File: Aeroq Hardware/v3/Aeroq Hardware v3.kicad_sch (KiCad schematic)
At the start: 63 parts, among them Q1 Si1308EDL, U2 ESP32-C3-MINI-1-N4, U3 AMS1117-3.3, U4 SCD40-D-R1

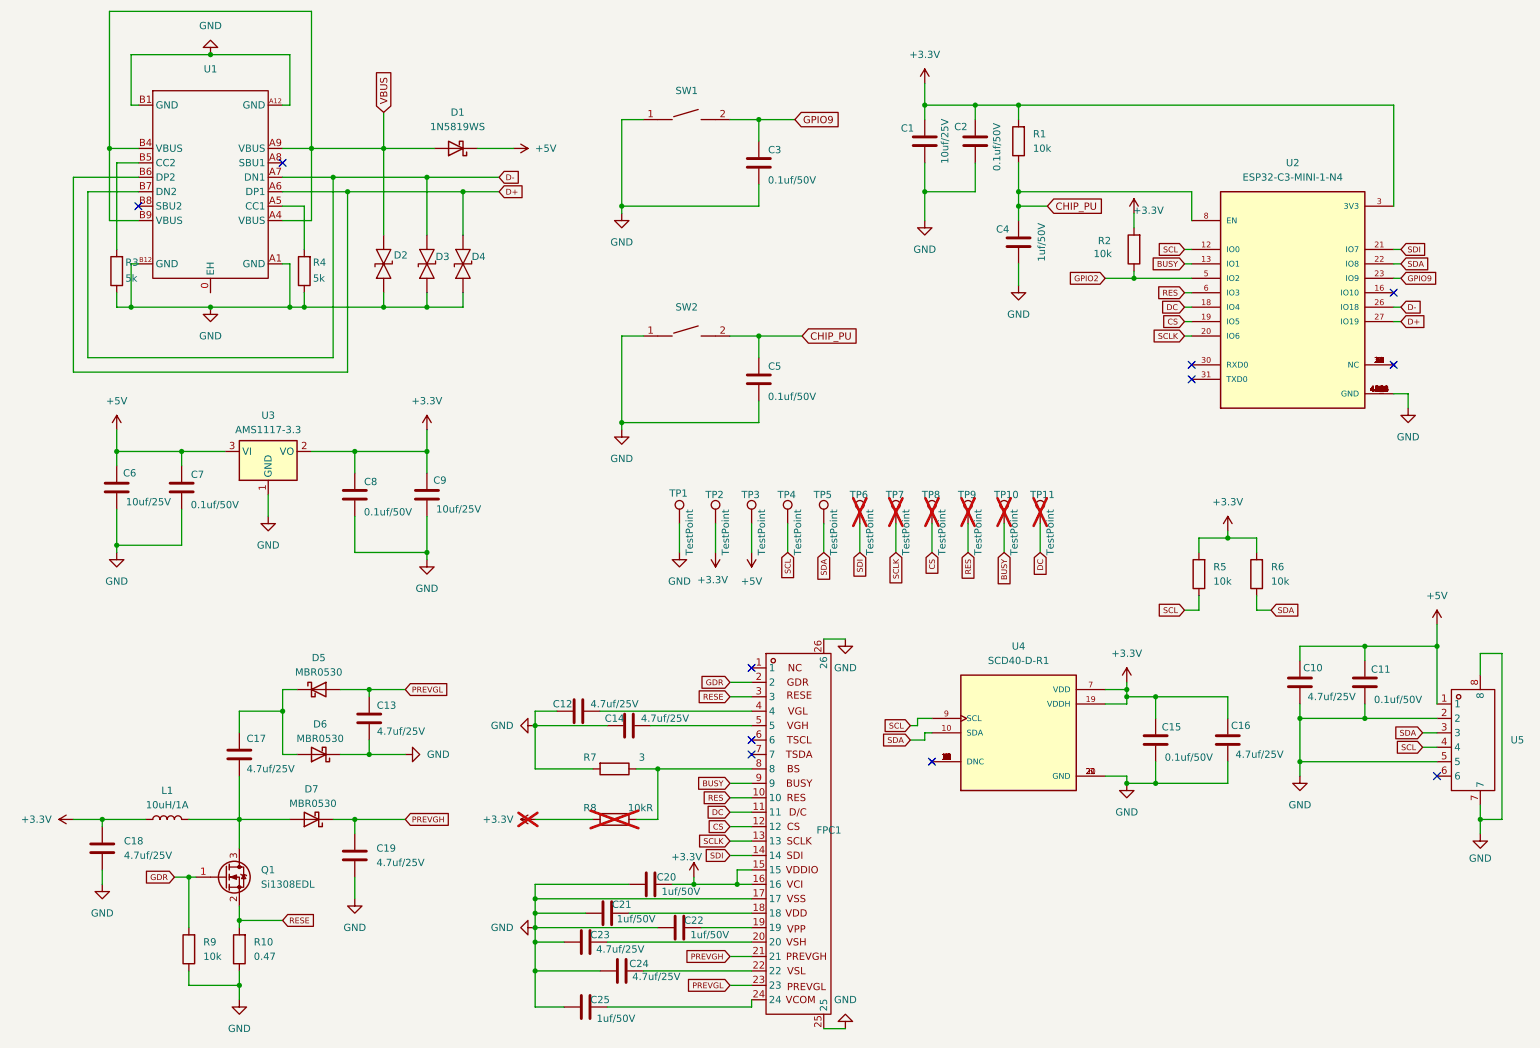
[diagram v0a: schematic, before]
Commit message: add my customizations
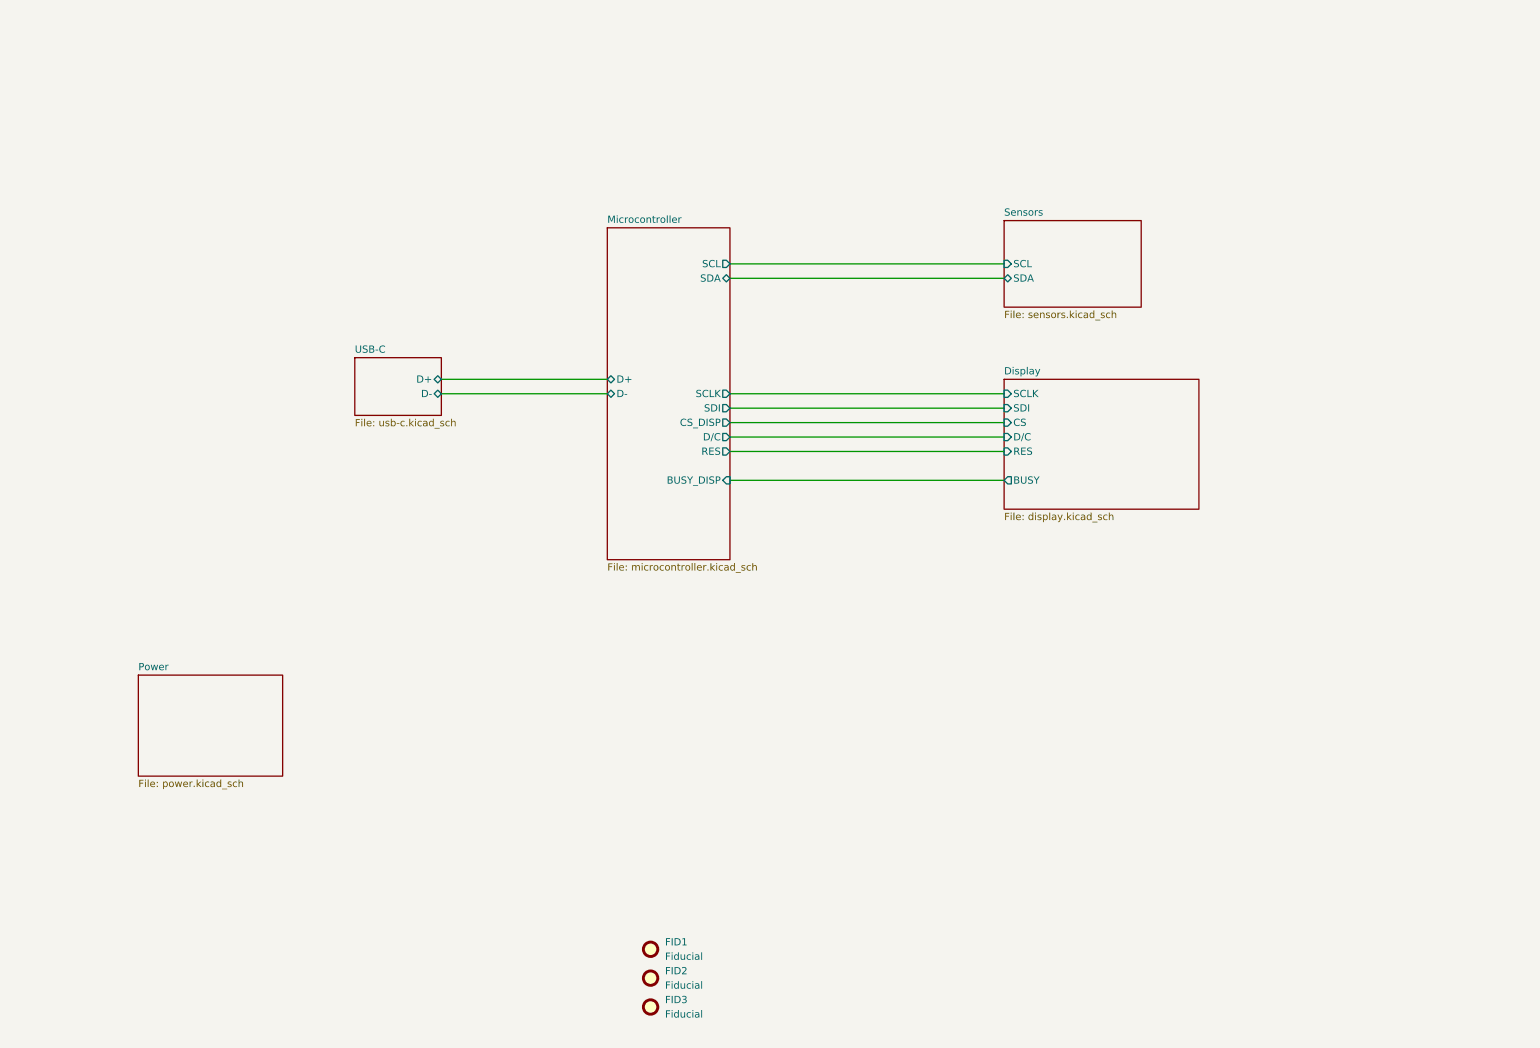
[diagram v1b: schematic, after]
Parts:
- removed C1, C6, C9: 10uf/25V, Capacitor_SMD:C_0603_1608Metric, symbol Device:C
- removed C10, C12, C13, C14, C16, C17, C18, C19, C23, C24: 4.7uf/25V, Capacitor_SMD:C_0603_1608Metric, symbol Device:C
- removed C11, C15, C2, C3, C5, C7, C8: 0.1uf/50V, Capacitor_SMD:C_0603_1608Metric, symbol Device:C
- removed C20, C21, C22, C25, C4: 1uf/50V, Capacitor_SMD:C_0603_1608Metric, symbol Device:C
- removed D1: 1N5819WS, Diode_SMD:D_SOD-323, symbol Diode:1N5819WS
- removed D2, D3, D4: ~, Project Footprints:SOD-523_L1.2-W0.8-LS1.6-BI, symbol LRC LESD5D5.0CT1G:LESD5D5.0CT1G
- removed D5, D6, D7: MBR0530, Diode_SMD:D_SOD-123, symbol Diode:MBR0530
- removed FPC1: ~, Project Footprints:FPC-SMD_24P-P0.50_FPC-05FB-24PH20, symbol FPC-05FB-24PH20:FPC-05FB-24PH20
- removed L1: 10uH/1A, Inductor_SMD:L_1210_3225Metric, symbol Device:L
- removed Q1: Si1308EDL, Package_TO_SOT_SMD:SOT-323_SC-70, symbol Transistor_FET:Si1308EDL
- removed R1, R2, R5, R6, R9: 10k, Resistor_SMD:R_0402_1005Metric, symbol Device:R
- removed R10: 0.47, Resistor_SMD:R_0402_1005Metric, symbol Device:R
- removed R3, R4: 5k, Resistor_SMD:R_0402_1005Metric, symbol Device:R
- removed R7: 3, Resistor_SMD:R_0402_1005Metric, symbol Device:R
- removed R8: 10kR, Resistor_SMD:R_0402_1005Metric, symbol Device:R
- removed SW1, SW2: ~, Project Footprints:SW-SMD_L3.9-W3.0-P4.45, symbol XUNPU TS-1088-AR02016:TS-1088-AR02016
- removed TP1, TP10, TP11, TP2, TP3, TP4, TP5, TP6, TP7, TP8, TP9: TestPoint, TestPoint:TestPoint_Pad_D1.5mm, symbol Connector:TestPoint
- removed U1: ~, Project Footprints:TYPE-C-SMD_USB4120-03-C, symbol TYPE-C 16PLT-H10:TYPE-C 16PLT-H10.0
- removed U2: ESP32-C3-MINI-1-N4, Project Footprints:XCVR_ESP32-C3-MINI-1-N4, symbol ESP32-C3-MINI-1-N4:ESP32-C3-MINI-1-N4
- removed U3: AMS1117-3.3, Package_TO_SOT_SMD:SOT-223-3_TabPin2, symbol Regulator_Linear:AMS1117-3.3
- removed U4: SCD40-D-R1, Project Footprints:XDCR_SCD40-D-R1, symbol SCD40-D-R1:SCD40-D-R1
- removed U5: ~, XUNPU WAFER-GH1.25-6PWB:CONN-SMD_6P-P1.25_XUNPU_WAFER-GH1.25-6PWB, symbol XUNPU WAFER-GH1.25-6PWB:WAFER-GH1.25-6PWB
- added FID1, FID2, FID3: Fiducial, Fiducial:Fiducial_0.5mm_Mask1.5mm, symbol 2s_mechanical:Fiducial 0.5 / 1.5
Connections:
- no-connect marks 11 -> 0
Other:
- added sheet Display (display.kicad_sch)
- added sheet Microcontroller (microcontroller.kicad_sch)
- added sheet Power (power.kicad_sch)
- added sheet Sensors (sensors.kicad_sch)
- added sheet USB-C (usb-c.kicad_sch)
